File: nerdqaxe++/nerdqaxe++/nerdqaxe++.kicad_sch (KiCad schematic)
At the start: 9 parts, among them J1 XT30

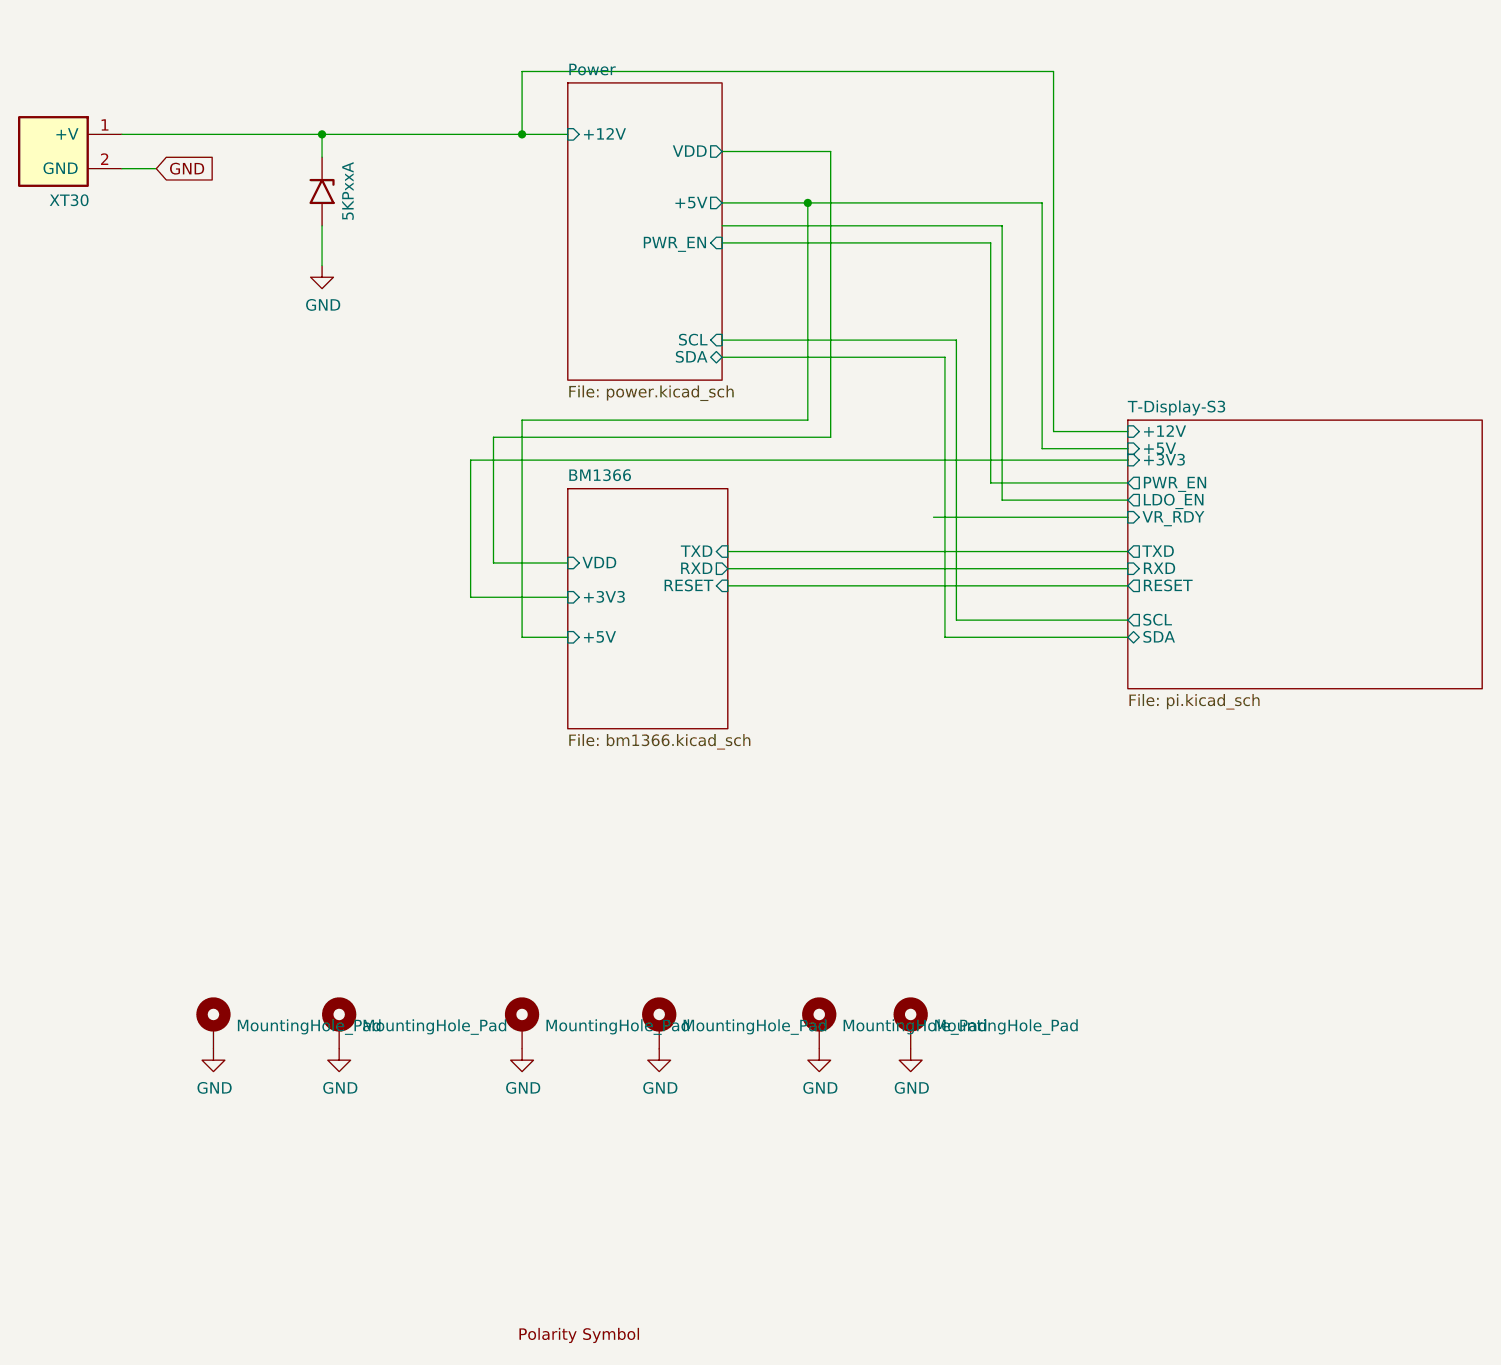
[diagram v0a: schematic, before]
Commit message: feature complete
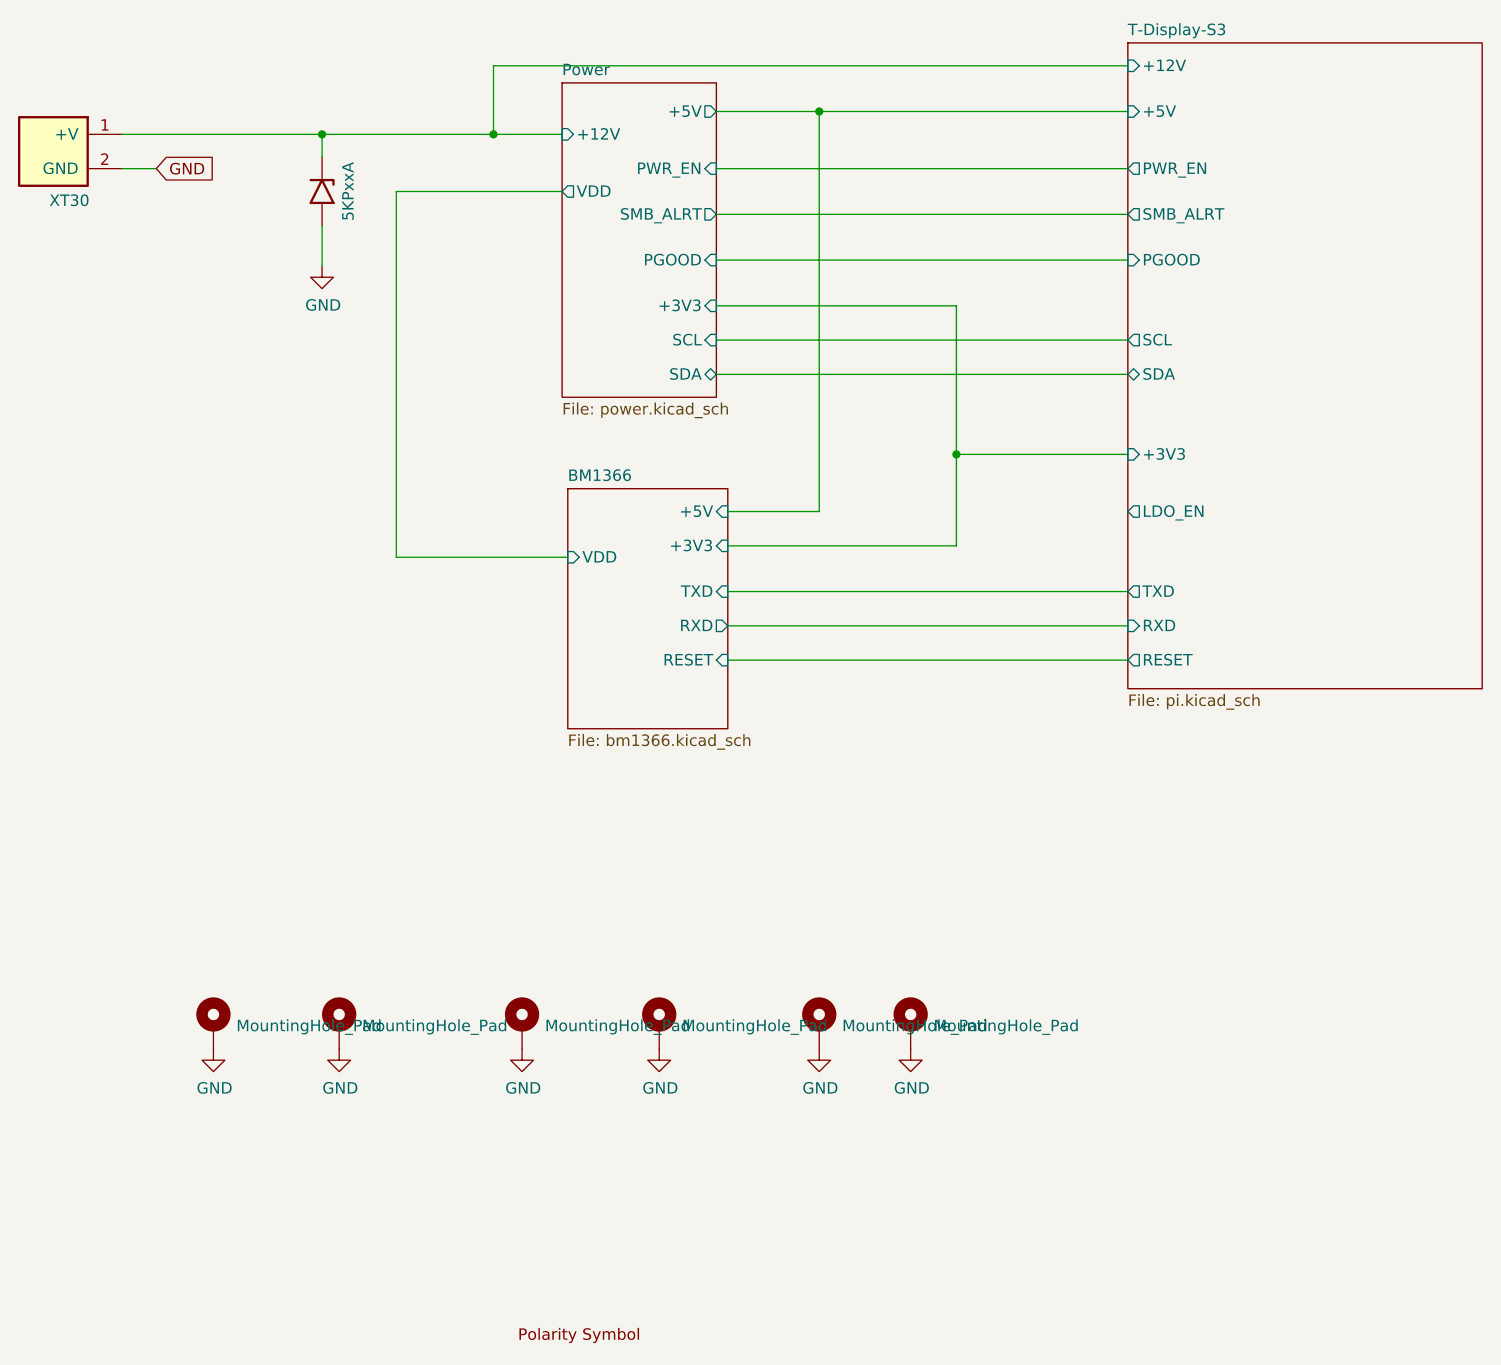
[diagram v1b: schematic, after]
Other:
- sheet Power ports: added +3V3, PGOOD, SMB_ALRT; removed none
- sheet T-Display-S3 ports: added PGOOD, SMB_ALRT; removed VR_RDY
